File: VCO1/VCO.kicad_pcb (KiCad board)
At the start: 2 copper layers, 78 parts, among them J10 Panel Power, J5 PANEL, J9 POWER, Q1 THAT340, Q2 2N3904, Q3 2N3904, U1 TL074, U2 TL072, U3 CA3080

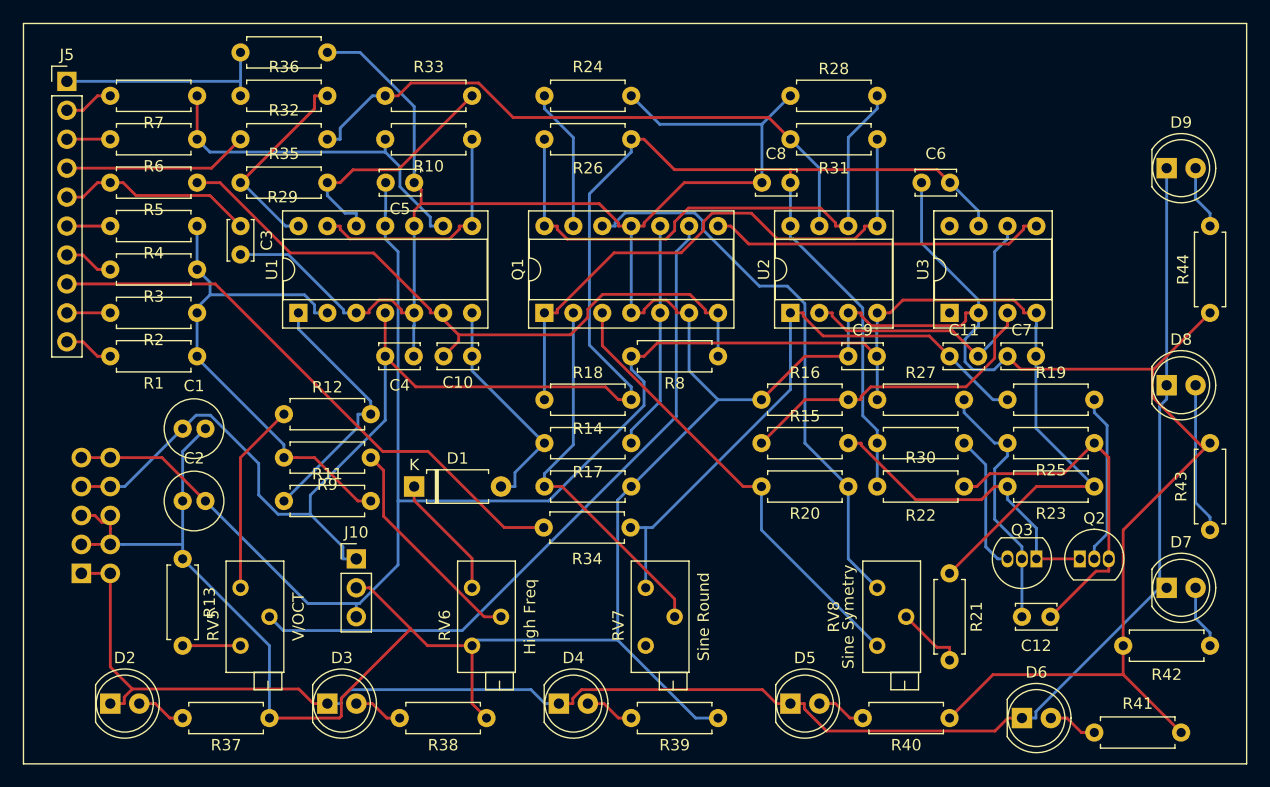
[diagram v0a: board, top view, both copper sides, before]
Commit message: update vco1 pcb
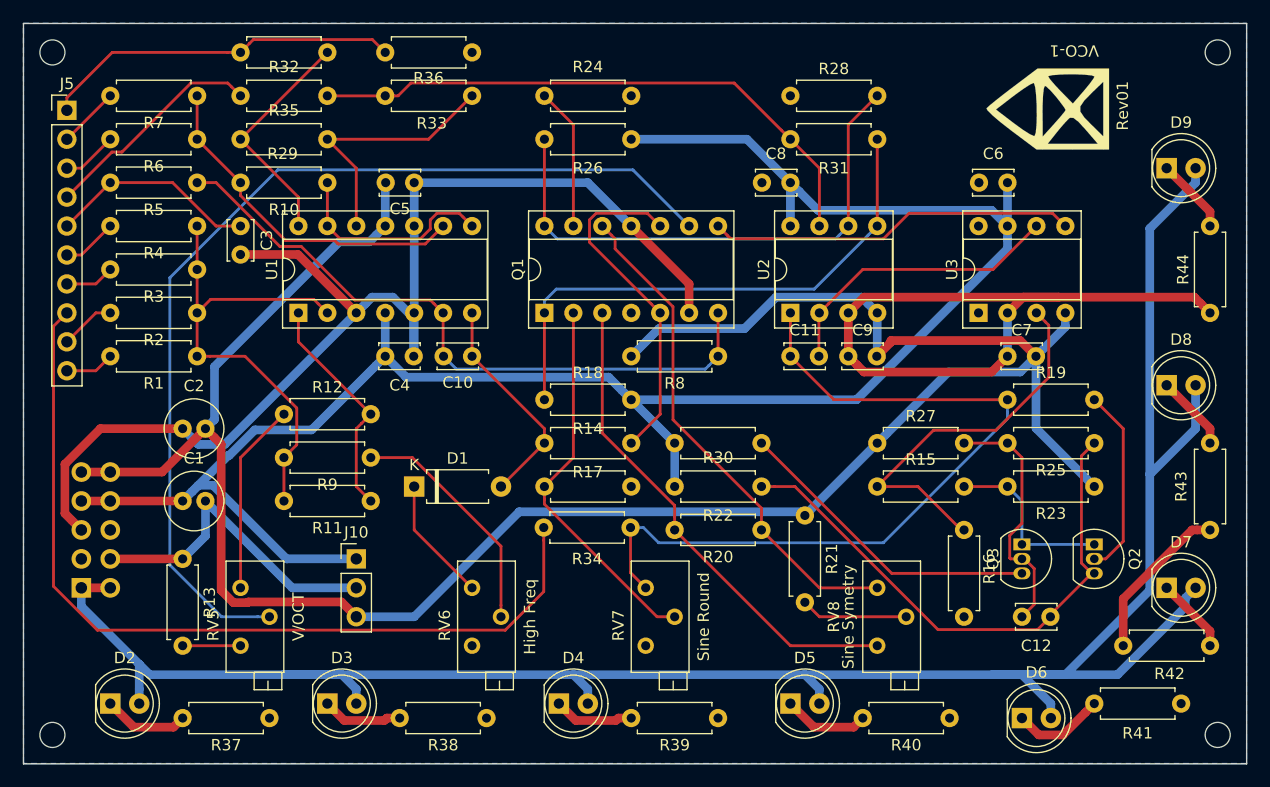
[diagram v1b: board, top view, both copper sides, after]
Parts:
- added G***: LOGO, logo:spielhuus, F.Cu at (149.6, 78.6)
- added REF**: MountingHole_2.2mm_M2_ISO7380, MountingHole:MountingHole_2.2mm_M2_ISO7380, F.Cu at (164.5, 133.6)
- added REF**: MountingHole_2.2mm_M2_ISO7380, MountingHole:MountingHole_2.2mm_M2_ISO7380, F.Cu at (62.2, 133.6)
- added REF**: MountingHole_2.2mm_M2_ISO7380, MountingHole:MountingHole_2.2mm_M2_ISO7380, F.Cu at (62.2, 73.7)
- added REF**: MountingHole_2.2mm_M2_ISO7380, MountingHole:MountingHole_2.2mm_M2_ISO7380, F.Cu at (164.5, 73.7)
- moved R16 26.1 mm to (142.2, 123.2), turned to 90 degrees
- moved R30 17.8 mm to (124.5, 108.0)
- moved R22 17.8 mm to (116.8, 111.8)
- moved C11 14.0 mm to (127.0, 100.3)
- moved R21 13.7 mm to (128.3, 114.3)
- moved R10 13.3 mm to (86.4, 85.1)
- moved R36 12.7 mm to (99.1, 73.7)
- moved R15 10.9 mm to (134.6, 111.8)
- moved R20 8.52 mm to (124.5, 115.6)
- moved R11 7.62 mm to (90.2, 113.0), turned to 180 degrees
- moved R43 7.62 mm to (163.8, 115.6), turned to 90 degrees
- moved C1 6.35 mm to (73.7, 113.0)
- moved C2 6.35 mm to (73.7, 106.7)
- moved C6 5.04 mm to (146.1, 85.1)
- moved R27 3.81 mm to (134.6, 108.0)
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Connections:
- D2 pad 1: +5V -> Net-(D2-Pad1)
- D2 pad 2: Net-(D2-Pad2) -> +5V
- D3 pad 1: +5V -> Net-(D3-Pad1)
- D3 pad 2: Net-(D3-Pad2) -> +5V
- D4 pad 1: +5V -> Net-(D4-Pad1)
- D4 pad 2: Net-(D4-Pad2) -> +5V
- D5 pad 1: +5V -> Net-(D5-Pad1)
- D5 pad 2: Net-(D5-Pad2) -> +5V
- D6 pad 1: +5V -> Net-(D6-Pad1)
- D6 pad 2: Net-(D6-Pad2) -> +5V
- D7 pad 1: +5V -> Net-(D7-Pad1)
- D7 pad 2: Net-(D7-Pad2) -> +5V
- D8 pad 1: +5V -> Net-(D8-Pad1)
- D8 pad 2: Net-(D8-Pad2) -> +5V
- D9 pad 1: +5V -> Net-(D9-Pad1)
- D9 pad 2: Net-(D9-Pad2) -> +5V
- R37 pad 2: Net-(D2-Pad2) -> Net-(D2-Pad1)
- R38 pad 2: Net-(D3-Pad2) -> Net-(D3-Pad1)
- R39 pad 2: Net-(D4-Pad2) -> Net-(D4-Pad1)
- R40 pad 2: Net-(D5-Pad2) -> Net-(D5-Pad1)
- R41 pad 2: Net-(D6-Pad2) -> Net-(D6-Pad1)
- R42 pad 2: Net-(D7-Pad2) -> Net-(D7-Pad1)
- R43 pad 2: Net-(D8-Pad2) -> Net-(D8-Pad1)
- R44 pad 2: Net-(D9-Pad2) -> Net-(D9-Pad1)
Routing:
- net GND: track 385.1 -> 209.8 mm
- net +5V: track 154.1 -> 195.4 mm
- net Net-(Q1-Pad9): track 61.2 -> 87.4 mm
- net /Triangle: track 50.7 -> 76.1 mm
- net -15V: track 178.0 -> 200.9 mm
- net Net-(C12-Pad2): track 31.5 -> 48.8 mm
- net Net-(C11-Pad1): track 53.4 -> 70.1 mm
- net Net-(Q3-Pad3): track 12.2 -> 27.6 mm
- net Net-(D8-Pad2): track 13.2 -> 0.00 mm
- net /Pulse: track 19.0 -> 31.6 mm
- net Net-(Q2-Pad1): track 27.8 -> 15.8 mm
- net Net-(Q1-Pad10): track 20.1 -> 30.1 mm
- net Net-(D6-Pad1): track 0.00 -> 8.10 mm
- net Net-(D5-Pad1): track 0.00 -> 7.54 mm
- net Net-(D2-Pad1): track 0.00 -> 7.54 mm
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- added copper zone on B.Cu, net GND
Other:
- board outline added: 107.3 x 65 mm
- board text added: "Rev01"
- board text added: "VCO-1"

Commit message: check pcb
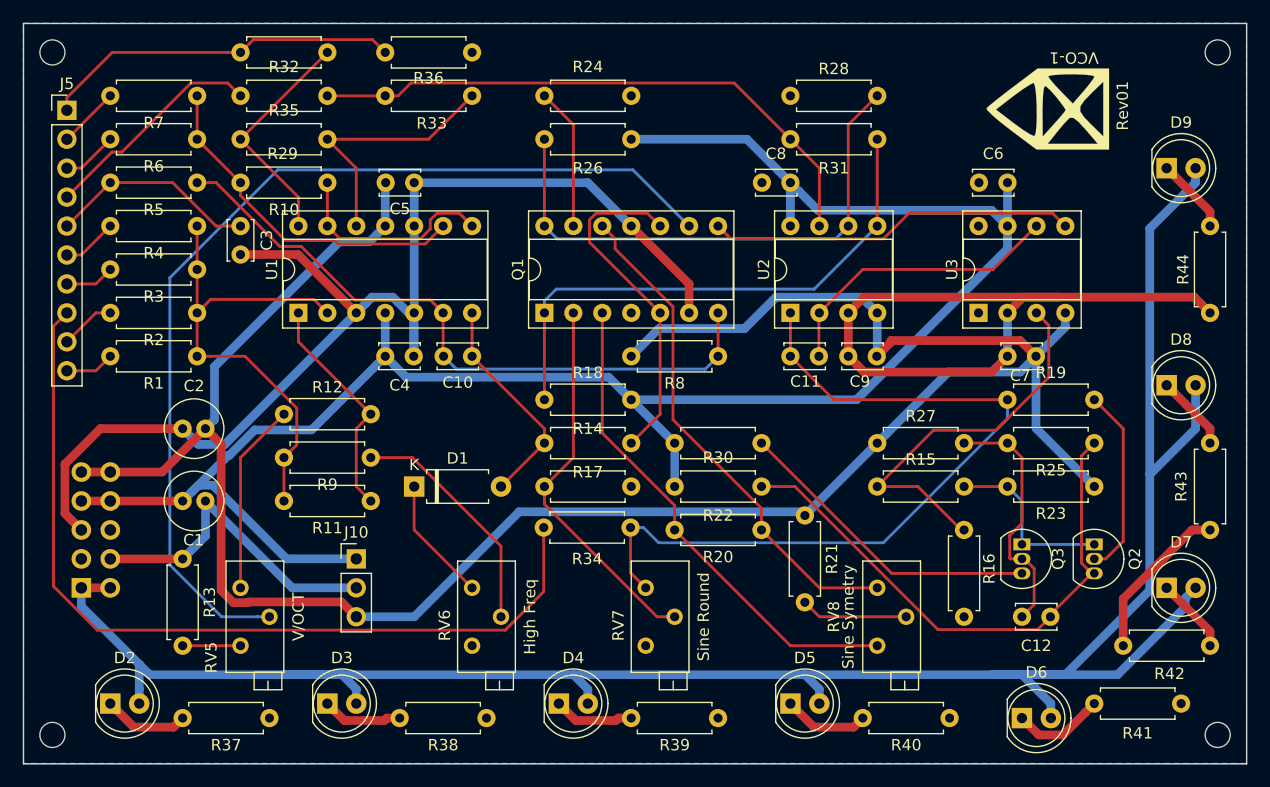
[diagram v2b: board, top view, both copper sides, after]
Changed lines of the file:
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@@
-(kicad_pcb (version 20171130) (host pcbnew 5.1.2)
+(kicad_pcb (version 20171130) (host pcbnew "(5.0.1)-4")
   (general
     (thickness 1.6)
@@
   (layers
     (0 F.Cu signal)
-    (31 B.Cu signal)
+    (31 B.Cu signal hide)
     (32 B.Adhes user)
     (33 F.Adhes user)
@@
   )
   (setup
-    (last_trace_width 0.762)
+    (last_trace_width 0.25)
     (user_trace_width 0.762)
     (user_trace_width 1.016)
@@
     (zone_45_only no)
     (trace_min 0.2)
+    (segment_width 0.2)
+    (edge_width 0.05)
     (via_size 0.8)
     (via_drill 0.4)
@@
     (uvia_min_size 0.2)
     (uvia_min_drill 0.1)
-    (edge_width 0.05)
-    (segment_width 0.2)
     (pcb_text_width 0.3)
     (pcb_text_size 1.5 1.5)
@@
     (solder_mask_min_width 0.25)
     (aux_axis_origin 0 0)
-    (visible_elements FFFFFF7F)
+    (visible_elements 7FFFFFFF)
     (pcbplotparams
       (layerselection 0x010fc_ffffffff)
@@
     (descr "Potentiometer, horizontal, Bourns 3296Z, https://www.bourns.com/pdfs/3296.pdf")
     (tags "Potentiometer horizontal Bourns 3296Z")
-    (fp_text reference RV5 (at -3.3 -2.4 90) (layer F.SilkS)
+    (fp_text reference RV5 (at -6.12 -2.57 90) (layer F.SilkS)
       (effects (font (size 1 1) (thickness 0.15)))
     )
@@
     (descr "C, Disc series, Radial, pin pitch=2.50mm, , diameter*width=3.4*2.1mm^2, Capacitor, http://www.vishay.com/docs/45233/krseries.pdf")
     (tags "C Disc series Radial pin pitch 2.50mm  diameter 3.4mm width 2.1mm Capacitor")
-    (fp_text reference C11 (at 1.25 -2.3) (layer F.SilkS)
+    (fp_text reference C11 (at 1.32 2.21) (layer F.SilkS)
       (effects (font (size 1 1) (thickness 0.15)))
     )
@@
     (descr "C, Disc series, Radial, pin pitch=2.50mm, , diameter*width=3.4*2.1mm^2, Capacitor, http://www.vishay.com/docs/45233/krseries.pdf")
     (tags "C Disc series Radial pin pitch 2.50mm  diameter 3.4mm width 2.1mm Capacitor")
-    (fp_text reference C9 (at 1.25 -2.3) (layer F.SilkS)
+    (fp_text reference C9 (at 1.02 2.21) (layer F.SilkS)
       (effects (font (size 1 1) (thickness 0.15)))
     )
@@
     (descr "C, Disc series, Radial, pin pitch=2.50mm, , diameter*width=3.4*2.1mm^2, Capacitor, http://www.vishay.com/docs/45233/krseries.pdf")
     (tags "C Disc series Radial pin pitch 2.50mm  diameter 3.4mm width 2.1mm Capacitor")
-    (fp_text reference C7 (at 1.25 -2.3) (layer F.SilkS)
+    (fp_text reference C7 (at 1.12 1.7) (layer F.SilkS)
       (effects (font (size 1 1) (thickness 0.15)))
     )
@@
     (descr "TO-92 leads in-line, narrow, oval pads, drill 0.75mm (see NXP sot054_po.pdf)")
     (tags "to-92 sc-43 sc-43a sot54 PA33 transistor")
-    (fp_text reference Q3 (at 1.27 2.54 90) (layer F.SilkS)
+    (fp_text reference Q3 (at 1.27 -3.175 90) (layer F.SilkS)
       (effects (font (size 1 1) (thickness 0.15)))
     )
@@
     (descr "C, Radial series, Radial, pin pitch=2.00mm, diameter=5mm, height=11mm, Non-Polar Electrolytic Capacitor")
     (tags "C Radial series Radial pin pitch 2.00mm diameter 5mm height 11mm Non-Polar Electrolytic Capacitor")
-    (fp_text reference C1 (at 1 -3.75) (layer F.SilkS)
+    (fp_text reference C1 (at 0.96 3.43) (layer F.SilkS)
       (effects (font (size 1 1) (thickness 0.15)))
     )
@@
     (effects (font (size 1 1) (thickness 0.15)))
   )
-  (gr_text VCO-1 (at 151.91 73.5 180) (layer F.SilkS)
+  (gr_text VCO-1 (at 151.89 74.12 180) (layer F.SilkS)
     (effects (font (size 1 1) (thickness 0.15)))
   )
